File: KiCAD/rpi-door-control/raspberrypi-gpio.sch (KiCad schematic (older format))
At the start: 24 parts, among them IC1 PC817, J1 RJ45, P1 CONN_13X2, P2 CONN_2, P3 CONN_2, P4 CONN_2, Q1 2N3904, Q2 PN2222A, SW1 SW_PUSH, U1 RELAY

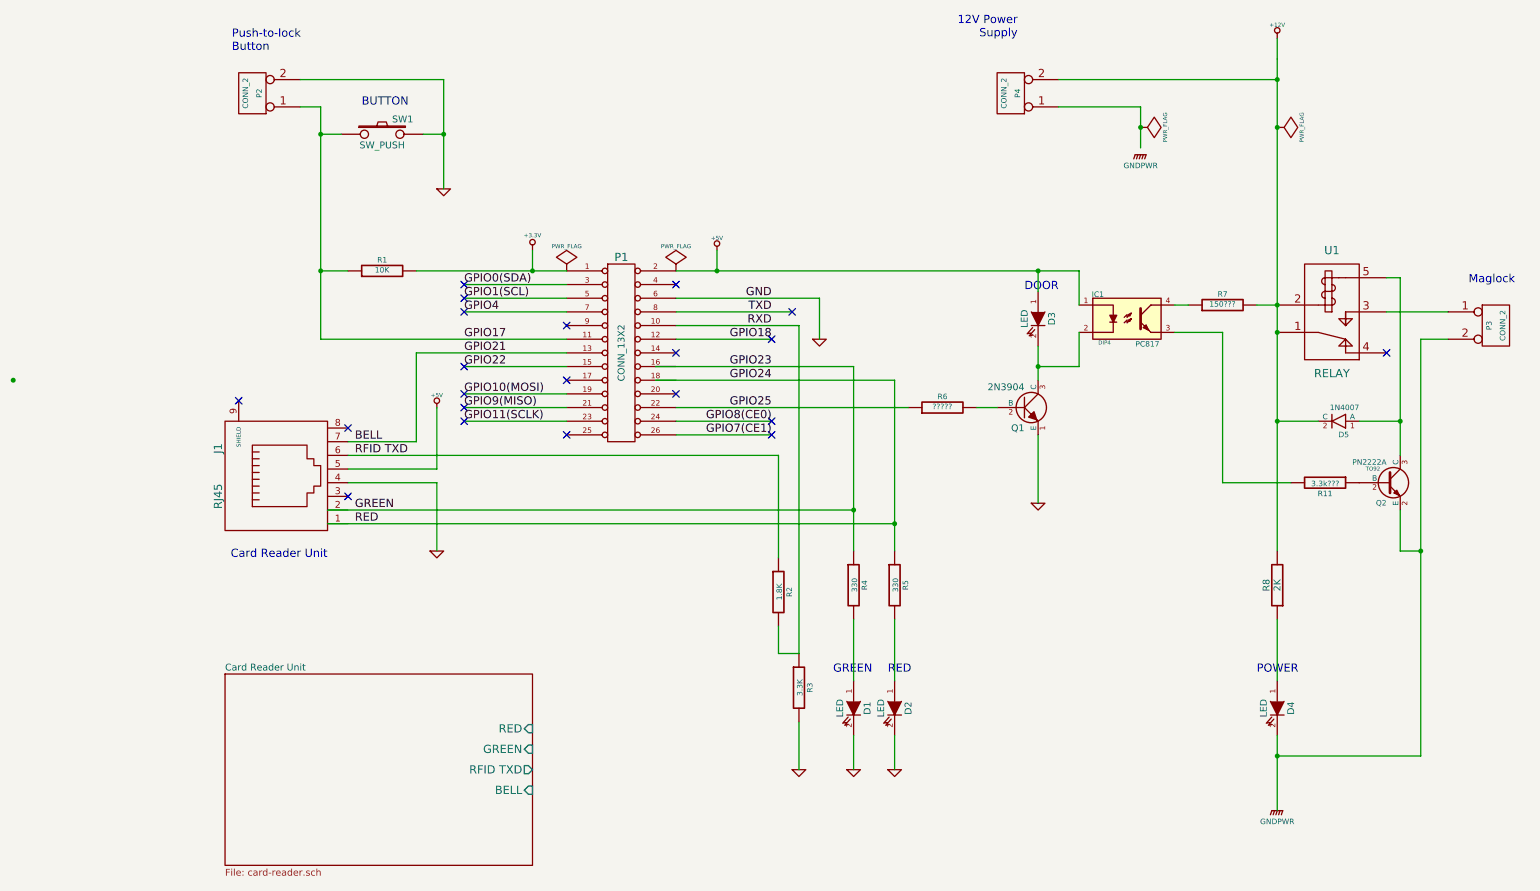
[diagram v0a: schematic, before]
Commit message: Created version 0.6
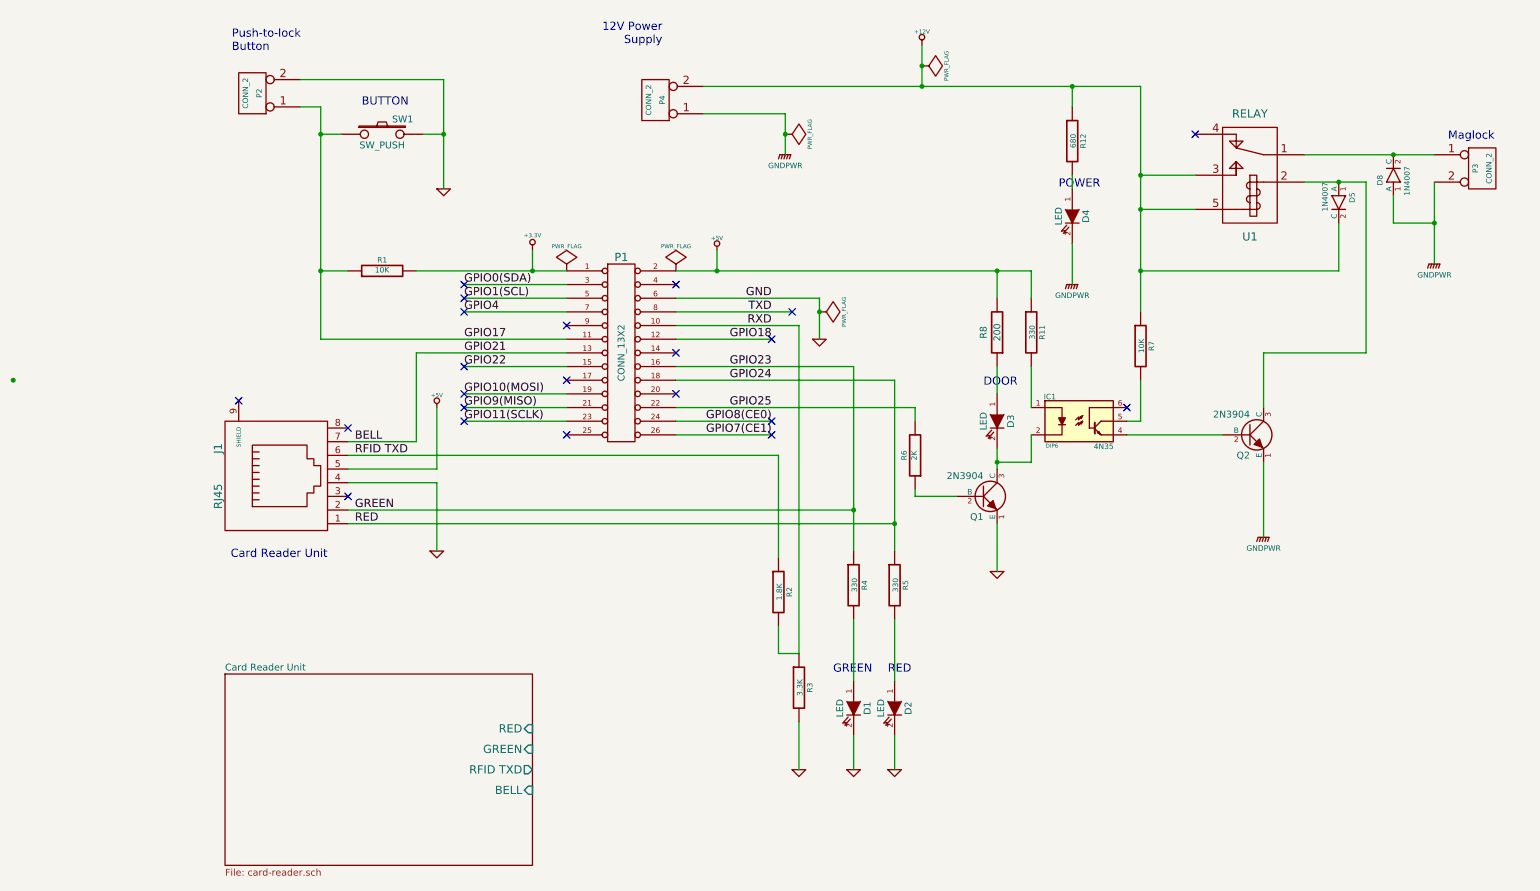
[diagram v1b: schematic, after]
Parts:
- removed IC1: PC817, DIP4, symbol PC817
- removed Q2: PN2222A, TO92, symbol PN2222A
- added D8: 1N4007, DO7, symbol 1N4004
- added IC1: 4N35, DIP6, symbol 4N35
- added Q2: 2N3904, ~, symbol NPN
- added R12: 680, ~, symbol R
- R11: value 3.3k??? -> 330
- R6: value ????? -> 2K
- R7: value 150??? -> 10K
- R8: value 2K -> 200
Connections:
- wire segments 96 -> 85
- no-connect marks 21 -> 22
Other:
- moved on the sheet: D3, D4, D5, P3, P4, Q1, R11, R6, R7, R8, U1
